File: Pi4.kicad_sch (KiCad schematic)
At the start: 6 parts, among them J601 Conn_02x02_Odd_Even, J602 Conn_02x02_Odd_Even, U601 RASPBERRY_PI_4B_4GB

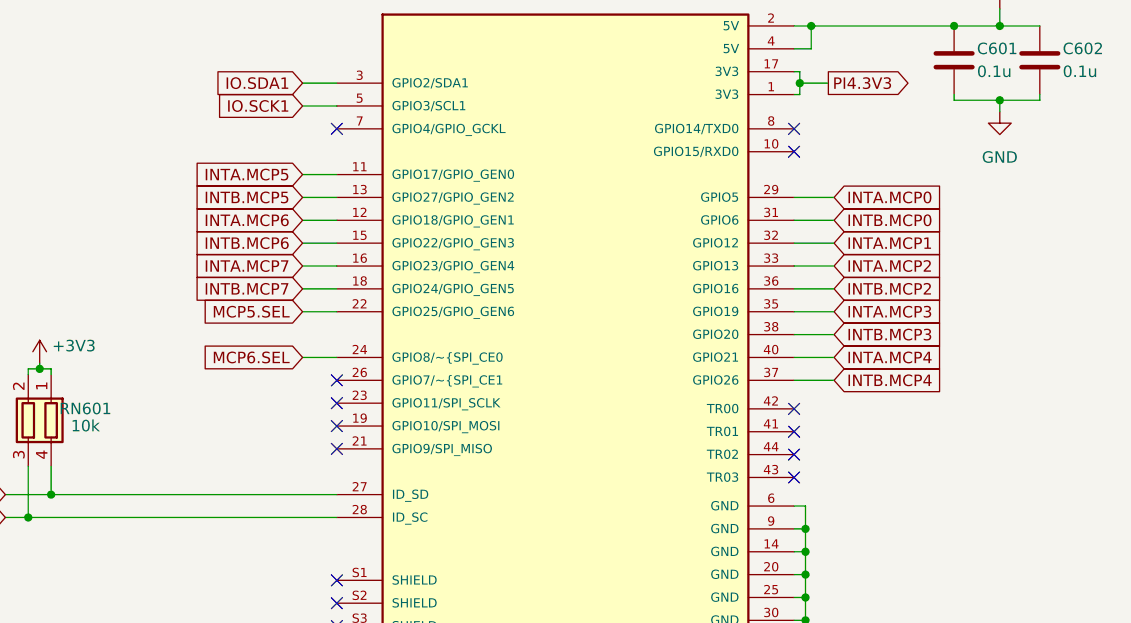
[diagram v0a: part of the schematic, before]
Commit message: Update 8/2
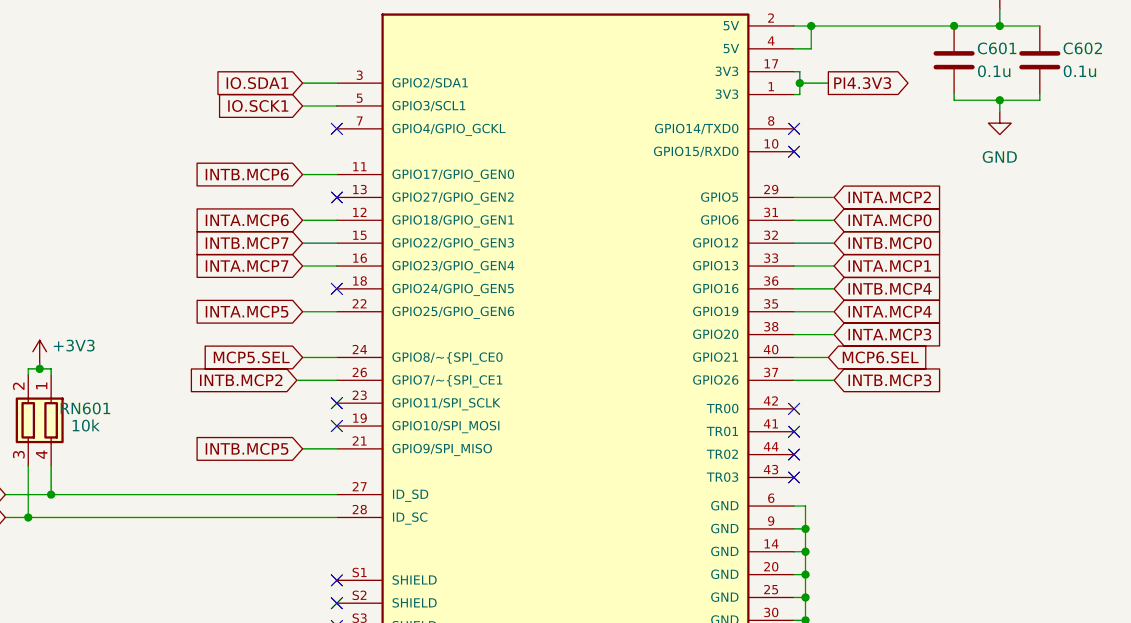
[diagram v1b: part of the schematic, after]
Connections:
- net INTA.MCP0: now also U601.31 (GPIO6); no longer U601.29 (GPIO5)
- net INTA.MCP1: now also U601.33 (GPIO13); no longer U601.32 (GPIO12)
- net INTA.MCP2: now also U601.29 (GPIO5); no longer U601.33 (GPIO13)
- net INTA.MCP3: now also U601.38 (GPIO20); no longer U601.35 (GPIO19)
- net INTA.MCP4: now also U601.35 (GPIO19); no longer U601.40 (GPIO21)
- net INTA.MCP5: now also U601.22 (GPIO25/GPIO_GEN6); no longer U601.11 (GPIO17/GPIO_GEN0)
- net INTB.MCP0: now also U601.32 (GPIO12); no longer U601.31 (GPIO6)
- net INTB.MCP2: now also U601.26 (GPIO7/~{SPI_CE1~{}); no longer U601.36 (GPIO16)
- net INTB.MCP3: now also U601.37 (GPIO26); no longer U601.38 (GPIO20)
- net INTB.MCP4: now also U601.36 (GPIO16); no longer U601.37 (GPIO26)
- net INTB.MCP5: now also U601.21 (GPIO9/SPI_MISO); no longer U601.13 (GPIO27/GPIO_GEN2)
- net INTB.MCP6: now also U601.11 (GPIO17/GPIO_GEN0); no longer U601.15 (GPIO22/GPIO_GEN3)
- net INTB.MCP7: now also U601.15 (GPIO22/GPIO_GEN3); no longer U601.18 (GPIO24/GPIO_GEN5)
- net MCP5.SEL: now also U601.24 (GPIO8/~{SPI_CE0~{}); no longer U601.22 (GPIO25/GPIO_GEN6)
- net MCP6.SEL: now also U601.40 (GPIO21); no longer U601.24 (GPIO8/~{SPI_CE0~{})
